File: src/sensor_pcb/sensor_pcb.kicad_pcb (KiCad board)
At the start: 4 copper layers, 67.6 x 56.9 mm, 113 parts, among them IC1 TCAN3414DRBR, J1 66200421024, J2 643280100305, J3 66200821024, J4 643280100305, J5 66200821024, J6 FTSH-107-02-L-DV, J7 66200421024, Q1 NPN BJT 40V 200mA, Q2 NPN BJT 40V 200mA, Q3 NPN BJT 40V 200mA, Q4 NPN BJT 40V 200mA, Q5 NPN BJT 40V 200mA, Q6 NPN BJT 40V 200mA, Q7 NPN BJT 40V 200mA, Q8 NPN BJT 40V 200mA, SW1 Button Switch SPST-No, U1 SHT45-AD1B, U2 16-bit ADC, U3 STM32L451CET6, U4 BMP581, Y1 16.0MHz

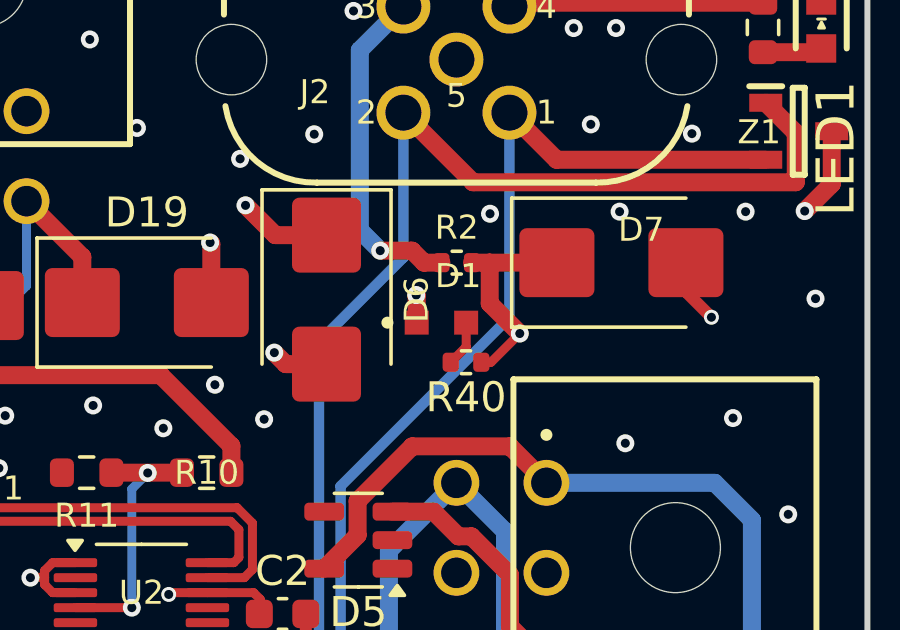
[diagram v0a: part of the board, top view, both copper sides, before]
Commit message: symbol update for spn
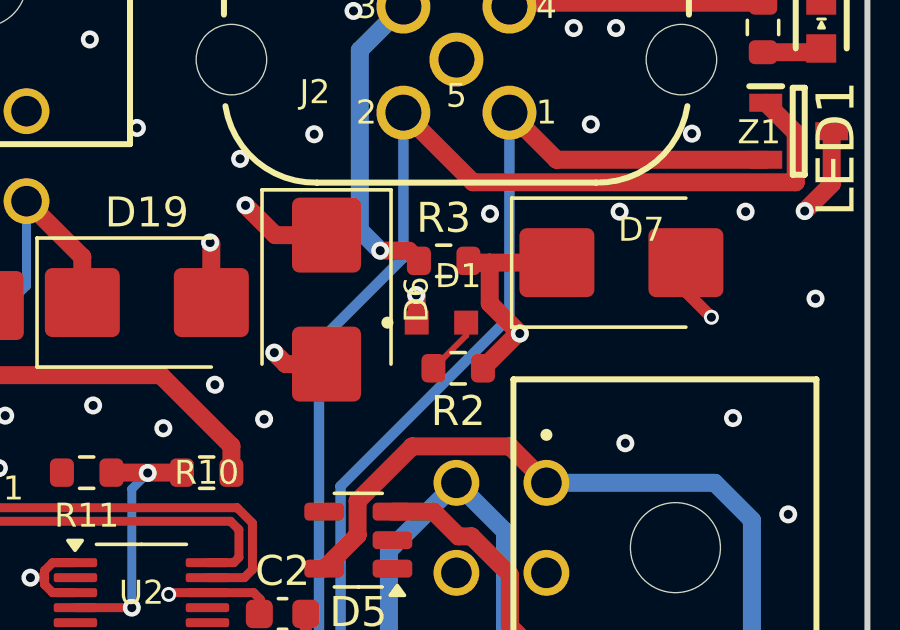
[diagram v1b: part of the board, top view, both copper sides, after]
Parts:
- removed R40: 100, Resistor_SMD:R_0402_1005Metric
- added R3: 100, Resistor_SMD:R_0603_1608Metric, F.Cu at (189.1, 68.9)
- R2: footprint Resistor_SMD:R_0402_1005Metric -> Resistor_SMD:R_0603_1608Metric
- moved R2 3.52 mm to (189.6, 72.5), turned to 180 degrees
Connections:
- R2 pad 1: Net-(J2-Pin_3) -> +3.3V
- R2 pad 2: +3.3V -> Net-(D1-PadA)
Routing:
- net Net-(J2-Pin_3): track 11.2 -> 10.4 mm
